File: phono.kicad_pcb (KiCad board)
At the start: 2 copper layers, 98.5 x 82 mm, 63 parts, among them J1 Power +30V, J2 R Phono in, J3 L Phono in, J4 R Phono out, J5 L Phono out, Q1 2N2222, Q2 2N2222, Q3 2N2222, Q4 2N2222, Q5 2N2222, Q6 2N2222

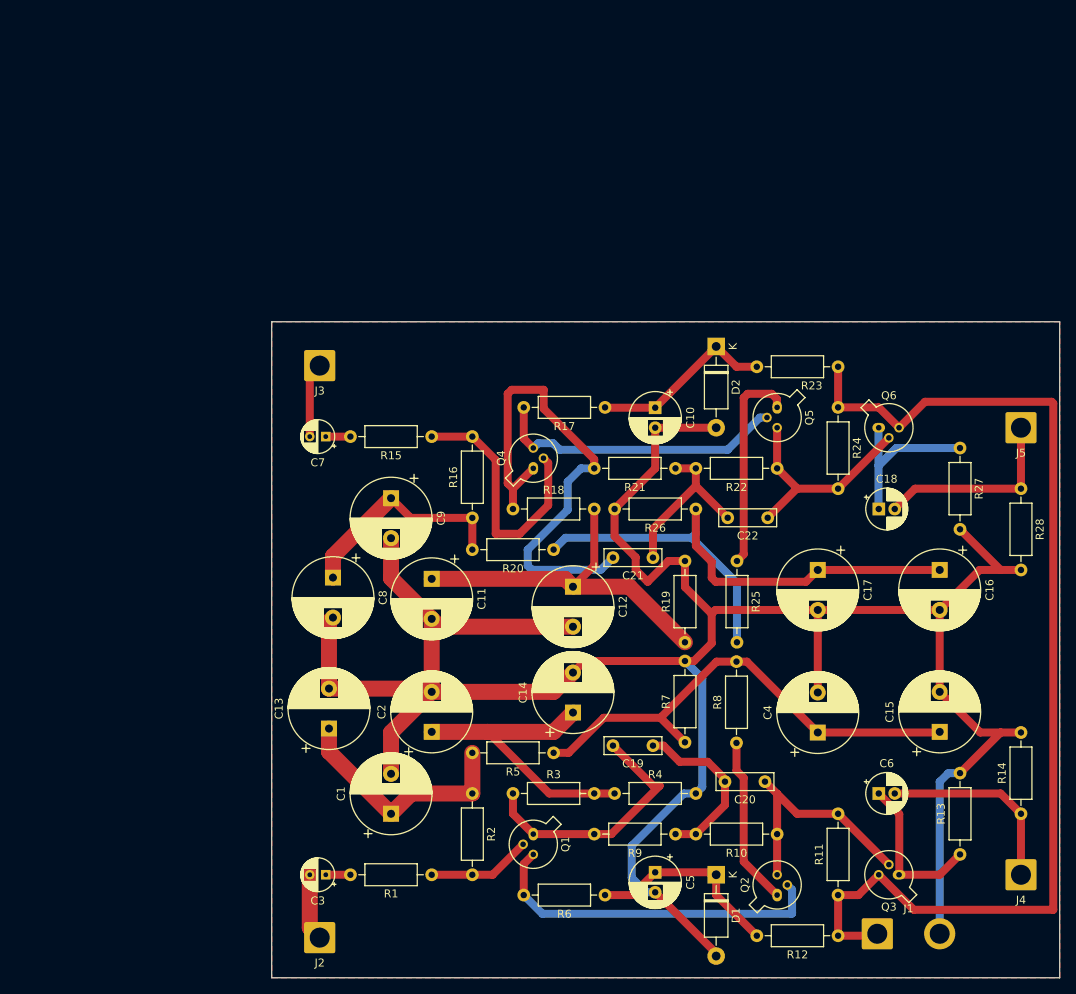
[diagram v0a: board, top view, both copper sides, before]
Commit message: Add files via upload
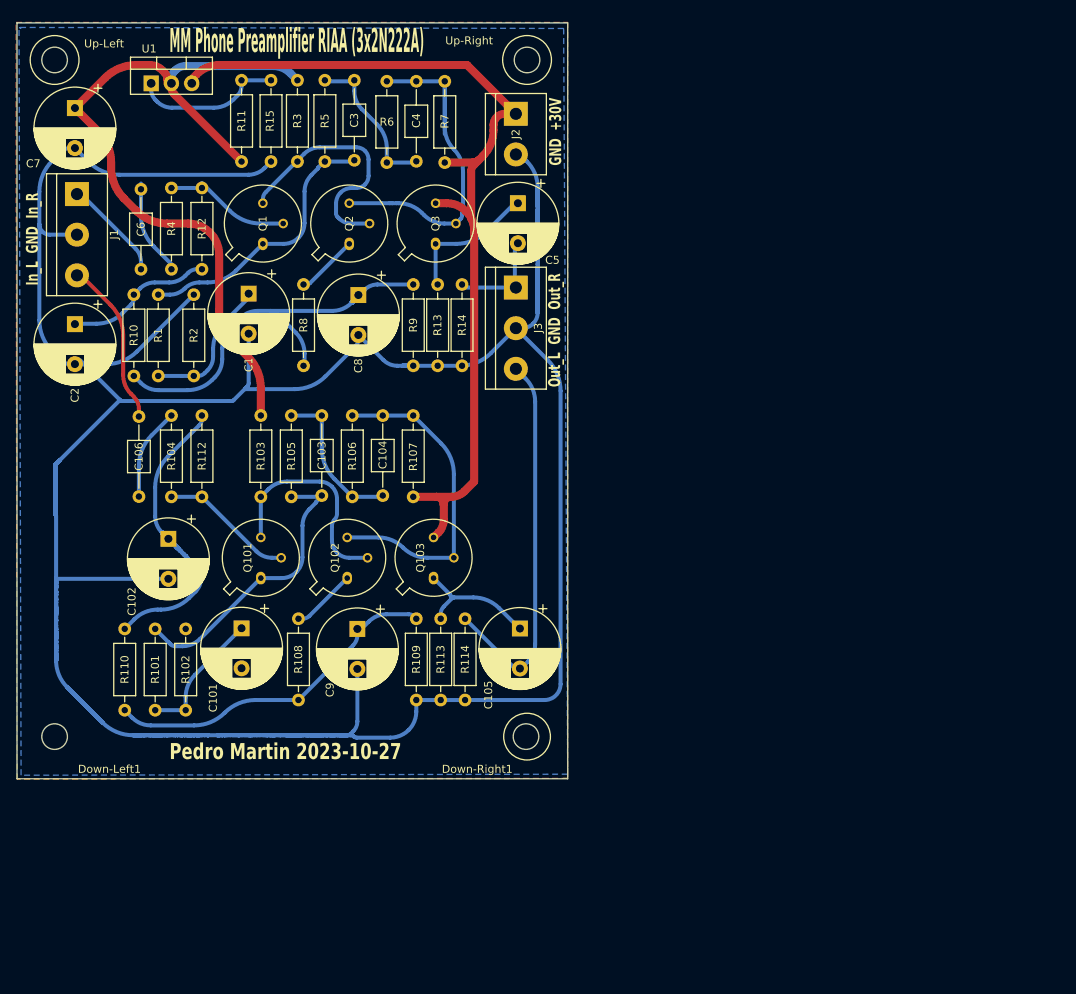
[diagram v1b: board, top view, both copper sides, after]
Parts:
- removed C10: 47uf, Capacitor_THT:CP_Radial_D6.3mm_P2.50mm
- removed C11, C12, C13, C14, C15, C16, C17: 150uf, Capacitor_THT:CP_Radial_D10.0mm_P5.00mm
- removed C18: 15uf, Capacitor_THT:CP_Radial_D5.0mm_P2.00mm
- removed C19, C21: 6.8nf, Capacitor_THT:C_Rect_L7.0mm_W2.0mm_P5.00mm
- removed C20, C22: 22nf, Capacitor_THT:C_Rect_L7.0mm_W2.0mm_P5.00mm
- removed D1, D2: 1N5250B, Diode_THT:D_DO-41_SOD81_P10.16mm_Horizontal
- removed J4: R Phono out, Connector_Wire:SolderWire-2sqmm_1x01_D2mm_OD3.9mm
- removed J5: L Phono out, Connector_Wire:SolderWire-2sqmm_1x01_D2mm_OD3.9mm
- removed Q4, Q5, Q6: 2N2222, Package_TO_SOT_THT:TO-18-3
- removed R16: 47k, Resistor_THT:R_Axial_DIN0207_L6.3mm_D2.5mm_P10.16mm_Horizontal
- removed R17: 8k2, Resistor_THT:R_Axial_DIN0207_L6.3mm_D2.5mm_P10.16mm_Horizontal
- removed R18: 150, Resistor_THT:R_Axial_DIN0207_L6.3mm_D2.5mm_P10.16mm_Horizontal
- removed R19, R26: 1k8, Resistor_THT:R_Axial_DIN0207_L6.3mm_D2.5mm_P10.16mm_Horizontal
- removed R20: 1k, Resistor_THT:R_Axial_DIN0207_L6.3mm_D2.5mm_P10.16mm_Horizontal
- removed R21: 12k, Resistor_THT:R_Axial_DIN0207_L6.3mm_D2.5mm_P10.16mm_Horizontal
- removed R22: 270k, Resistor_THT:R_Axial_DIN0207_L6.3mm_D2.5mm_P10.16mm_Horizontal
- removed R23: 680, Resistor_THT:R_Axial_DIN0207_L6.3mm_D2.5mm_P10.16mm_Horizontal
- removed R24: 6k, Resistor_THT:R_Axial_DIN0207_L6.3mm_D2.5mm_P10.16mm_Horizontal
- removed R25: 100, Resistor_THT:R_Axial_DIN0207_L6.3mm_D2.5mm_P10.16mm_Horizontal
- removed R27: 4k7, Resistor_THT:R_Axial_DIN0207_L6.3mm_D2.5mm_P10.16mm_Horizontal
- removed R28: 10k, Resistor_THT:R_Axial_DIN0207_L6.3mm_D2.5mm_P10.16mm_Horizontal
- added C101: 300u, Capacitor_THT:CP_Radial_D10.0mm_P5.00mm, F.Cu at (86.2, 96.3)
- added C102: 300u, Capacitor_THT:CP_Radial_D10.0mm_P5.00mm, F.Cu at (77.1, 85.1)
- added C103: 6n8, Capacitor_THT:C_Axial_L3.8mm_D2.6mm_P10.00mm_Horizontal, F.Cu at (96.3, 79.7)
- added C104: 22n, Capacitor_THT:C_Axial_L3.8mm_D2.6mm_P10.00mm_Horizontal, F.Cu at (103.9, 79.7)
- added C105: 47u, Capacitor_THT:CP_Radial_D10.0mm_P5.00mm, F.Cu at (121.0, 96.3)
- added C106: 1uF, Capacitor_THT:C_Axial_L3.8mm_D2.6mm_P10.00mm_Horizontal, F.Cu at (73.4, 69.8)
- added Down-Left1: MountingHole_3.2mm_M3, MountingHole:MountingHole_3.2mm_M3, F.Cu at (62.9, 109.9)
- added Down-Right1: MountingHole_3.2mm_M3, MountingHole:MountingHole_3.2mm_M3, F.Cu at (121.8, 109.9)
- added Q101: 2N2222, Package_TO_SOT_THT:TO-39-3, F.Cu at (88.6, 90.0)
- added Q102: 2N2222, Package_TO_SOT_THT:TO-39-3, F.Cu at (99.4, 90.0)
- added Q103: 2N2222, Package_TO_SOT_THT:TO-39-3, F.Cu at (110.2, 90.0)
- added R101: 150, Resistor_THT:R_Axial_DIN0207_L6.3mm_D2.5mm_P10.16mm_Horizontal, F.Cu at (75.4, 96.4)
- added R102: 1K8, Resistor_THT:R_Axial_DIN0207_L6.3mm_D2.5mm_P10.16mm_Horizontal, F.Cu at (79.2, 106.6)
- added R103: 8K2, Resistor_THT:R_Axial_DIN0207_L6.3mm_D2.5mm_P10.16mm_Horizontal, F.Cu at (88.6, 69.7)
- added R104: 100, Resistor_THT:R_Axial_DIN0207_L6.3mm_D2.5mm_P10.16mm_Horizontal, F.Cu at (77.5, 69.7)
- added R105: 12K, Resistor_THT:R_Axial_DIN0207_L6.3mm_D2.5mm_P10.16mm_Horizontal, F.Cu at (92.5, 79.9)
- added R106: 270K, Resistor_THT:R_Axial_DIN0207_L6.3mm_D2.5mm_P10.16mm_Horizontal, F.Cu at (100.1, 79.9)
- added R107: 6K, Resistor_THT:R_Axial_DIN0207_L6.3mm_D2.5mm_P10.16mm_Horizontal, F.Cu at (107.7, 79.9)
- added R108: 100, Resistor_THT:R_Axial_DIN0207_L6.3mm_D2.5mm_P10.16mm_Horizontal, F.Cu at (93.3, 95.1)
- added R109: 1K8, Resistor_THT:R_Axial_DIN0207_L6.3mm_D2.5mm_P10.16mm_Horizontal, F.Cu at (108.1, 95.1)
- added R110: 1K, Resistor_THT:R_Axial_DIN0207_L6.3mm_D2.5mm_P10.16mm_Horizontal, F.Cu at (71.6, 96.4)
- added R112: 47K, Resistor_THT:R_Axial_DIN0207_L6.3mm_D2.5mm_P10.16mm_Horizontal, F.Cu at (81.3, 79.9)
- added R113: 4K7, Resistor_THT:R_Axial_DIN0207_L6.3mm_D2.5mm_P10.16mm_Horizontal, F.Cu at (111.1, 95.1)
- added R114: 10K, Resistor_THT:R_Axial_DIN0207_L6.3mm_D2.5mm_P10.16mm_Horizontal, F.Cu at (114.2, 95.1)
- added U1: LM317_TO-220, Package_TO_SOT_THT:TO-220-3_Vertical, F.Cu at (74.9, 28.2)
- added Up-Left: MountingHole_3.2mm_M3, MountingHole:MountingHole_3.2mm_M3, F.Cu at (62.9, 25.3)
- added Up-Right: MountingHole_3.2mm_M3, MountingHole:MountingHole_3.2mm_M3, F.Cu at (121.9, 25.3)
- C1, C2, C8, C9: value 150uf -> 300u
- C3: value 1uf -> 6n8; footprint Capacitor_THT:CP_Radial_D4.0mm_P2.00mm -> Capacitor_THT:C_Axial_L3.8mm_D2.6mm_P10.00mm_Horizontal
- C4: value 150uf -> 22n; footprint Capacitor_THT:CP_Radial_D10.0mm_P5.00mm -> Capacitor_THT:C_Axial_L3.8mm_D2.6mm_P10.00mm_Horizontal
- C5: value 47uf -> 47u; footprint Capacitor_THT:CP_Radial_D6.3mm_P2.50mm -> Capacitor_THT:CP_Radial_D10.0mm_P5.00mm
- C6: value 15uf -> 1uF; footprint Capacitor_THT:CP_Radial_D5.0mm_P2.00mm -> Capacitor_THT:C_Axial_L3.8mm_D2.6mm_P10.00mm_Horizontal
- C7: value 1uf -> 47u; footprint Capacitor_THT:CP_Radial_D4.0mm_P2.00mm -> Capacitor_THT:CP_Radial_D10.0mm_P5.00mm
- J1: value Power +30V -> Conn_01x03_Pin; footprint Connector_Wire:SolderWire-2sqmm_1x02_P7.8mm_D2mm_OD3.9mm -> TerminalBlock:TerminalBlock_bornier-3_P5.08mm
- J2: value R Phono in -> Conn_01x02_Pin; footprint Connector_Wire:SolderWire-2sqmm_1x01_D2mm_OD3.9mm -> TerminalBlock:TerminalBlock_bornier-2_P5.08mm
- J3: value L Phono in -> Conn_01x03_Pin; footprint Connector_Wire:SolderWire-2sqmm_1x01_D2mm_OD3.9mm -> TerminalBlock:TerminalBlock_bornier-3_P5.08mm
- Q1, Q2, Q3: footprint Package_TO_SOT_THT:TO-18-3 -> Package_TO_SOT_THT:TO-39-3
- R1: value 100 -> 150
- R10: value 270k -> 1K
- R11: value 6k -> 1K
- R12: value 680 -> 47K
- R13: value 4k7 -> 4K7
- R14: value 10k -> 10K
- R15: value 100 -> 15K
- R2: value 47k -> 1K8
- R3: value 150 -> 8K2
- R4: value 1k8 -> 100
- R5: value 1k -> 12K
- R6: value 8k2 -> 270K
- R7: value 1k8 -> 6K
- R9: value 12k -> 1K8
- moved J1 136.2 mm to (65.7, 42.0), turned to -90 degrees
- moved R12 122.7 mm to (81.3, 41.3), turned to -90 degrees
- moved R11 118.2 mm to (86.2, 38.0)
- moved C6 113.1 mm to (73.7, 51.4), turned to 90 degrees
- moved J2 105.9 mm to (120.5, 32.0), turned to -90 degrees
- moved R10 104.9 mm to (72.8, 54.6), turned to -90 degrees
- moved Q3 97.9 mm to (110.5, 48.3), turned to 90 degrees
- moved Q2 97.4 mm to (99.7, 48.3)
- moved R13 96.6 mm to (110.7, 53.3), turned to -90 degrees
- moved R14 96.2 mm to (113.8, 53.3), turned to -90 degrees
- moved R6 95.5 mm to (104.4, 38.1), turned to 90 degrees
- moved R3 93.1 mm to (93.2, 27.8), turned to -90 degrees
- moved C3 89.4 mm to (100.3, 37.8), turned to 90 degrees
- moved R7 87.9 mm to (111.6, 27.9), turned to -90 degrees
- moved C4 87.3 mm to (108.1, 37.9)
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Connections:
- C2 pad 1: Net-(C14-Pad1) -> Net-(C2-Pad1)
- C3 pad 1: Net-(C3-Pad1) -> Net-(Q1-E)
- C3 pad 2: Net-(J2-Pin_1) -> Net-(C3-Pad2)
- C4 pad 1: Net-(C15-Pad1) -> Net-(C3-Pad2)
- C4 pad 2: GND -> Net-(Q2-C)
- C5 pad 1: Net-(D1-K) -> Net-(Q3-E)
- C5 pad 2: GND -> Output-R
- C6 pad 1: Net-(Q3-E) -> Input-R
- C6 pad 2: Net-(J4-Pin_1) -> Net-(C6-Pad2)
- C7 pad 1: Net-(C7-Pad1) -> +20V
- C7 pad 2: Net-(J3-Pin_1) -> GND
- C9 pad 1: Net-(C8-Pad1) -> Net-(C9-Pad1)
- J1 pad 1: +28V -> Input-R
- J2 pad 1: Net-(J2-Pin_1) -> +28V
- J3 pad 1: Net-(J3-Pin_1) -> Output-R
- R1 pad 1: Net-(Q1-B) -> Net-(Q1-E)
- R1 pad 2: Net-(C3-Pad1) -> Net-(C1-Pad1)
- R10 pad 1: Net-(Q2-C) -> Net-(C2-Pad1)
- R10 pad 2: Net-(C19-Pad1) -> Net-(C8-Pad1)
- R11 pad 1: +28V -> +20V
- R11 pad 2: Net-(Q2-C) -> Net-(U1-ADJ)
- R12 pad 1: +28V -> Net-(Q1-B)
- R12 pad 2: Net-(D1-K) -> Net-(C2-Pad1)
- R14 pad 1: Net-(J4-Pin_1) -> Output-R
- R15 pad 1: Net-(Q4-B) -> Net-(U1-ADJ)
- R15 pad 2: Net-(C7-Pad1) -> GND
- R2 pad 2: Net-(Q1-B) -> GND
- R3 pad 1: Net-(Q1-E) -> +20V
- R3 pad 2: Net-(C14-Pad1) -> Net-(Q1-C)
- R4 pad 1: Net-(C14-Pad1) -> Net-(C6-Pad2)
- R4 pad 2: GND -> Net-(Q1-B)
- R5 pad 1: Net-(C15-Pad1) -> Net-(Q1-E)
- R5 pad 2: Net-(C1-Pad1) -> Net-(C3-Pad2)
- R6 pad 1: Net-(D1-K) -> Net-(C3-Pad2)
- R6 pad 2: Net-(Q1-C) -> Net-(Q2-C)
- R7 pad 1: Net-(C15-Pad1) -> Net-(Q2-C)
- R7 pad 2: GND -> +28V
- R8 pad 2: Net-(C15-Pad1) -> Net-(C8-Pad1)
- R9 pad 1: Net-(C19-Pad1) -> Net-(C8-Pad1)
- R9 pad 2: Net-(Q1-E) -> GND
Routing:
- net +20V: track 0.00 -> 96.2 mm
- net Net-(C16-Pad1): track 75.8 -> 0.00 mm
- net Net-(Q4-E): track 63.5 -> 0.00 mm
- net Net-(C15-Pad1): track 61.0 -> 0.00 mm
- net Output-L: track 0.00 -> 47.7 mm
- net Net-(C11-Pad1): track 45.8 -> 0.00 mm
- net Net-(C9-Pad1): track 0.00 -> 42.2 mm
- net Net-(Q102-C): track 0.00 -> 41.2 mm
- net Net-(C14-Pad1): track 37.7 -> 0.00 mm
- net GND: track 316.9 -> 354.3 mm
- net Net-(Q4-C): track 37.0 -> 0.00 mm
- net Net-(Q101-E): track 0.00 -> 36.3 mm
- net Net-(C102-Pad1): track 0.00 -> 34.3 mm
- net Net-(Q4-B): track 32.6 -> 0.00 mm
- net Net-(Q5-C): track 28.0 -> 0.00 mm
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- added copper zone on B.Cu, net GND
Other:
- board size 98.5 x 82 mm -> 68.8 x 94.5 mm
- board text added: "GND +30V"
- board text added: "In_L GND In_R"
- board text added: "MM Phone Preamplifier RIAA (3x2N222A)"
- board text added: "Out_L GND Out_R"
- board text added: "Pedro Martin 2023-10-27"
